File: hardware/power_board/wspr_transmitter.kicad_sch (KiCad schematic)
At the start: 3 parts, among them J6 Conn_Coaxial_Small, J7 Conn_Coaxial_Small, Y2 Si5351A-B-GT

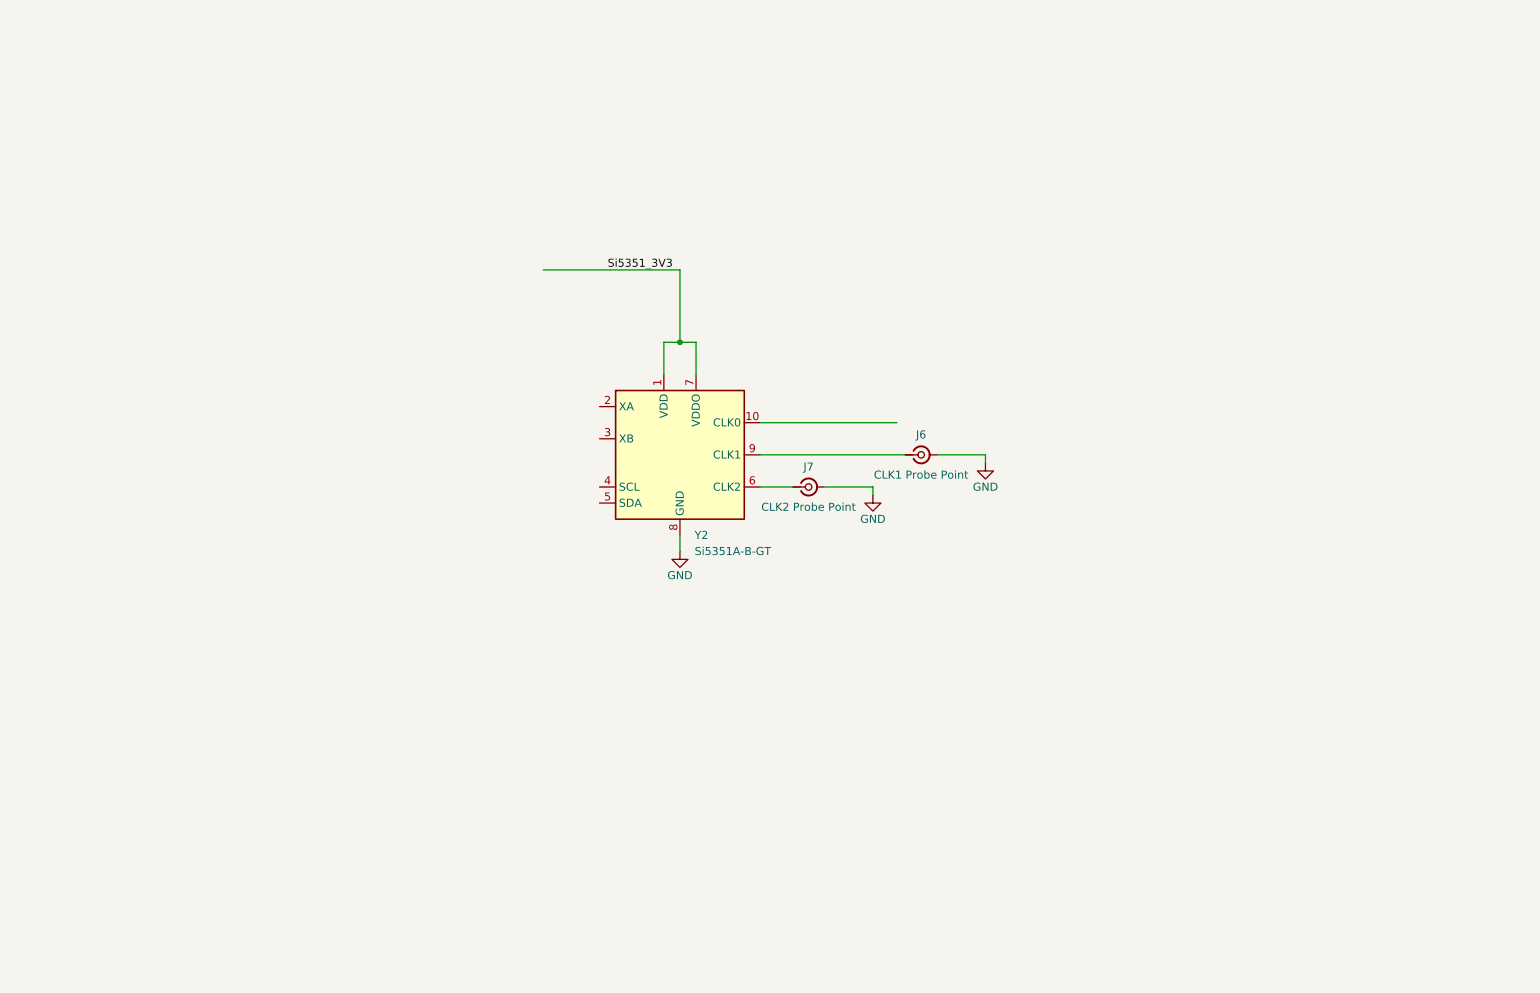
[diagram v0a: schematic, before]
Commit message: sync
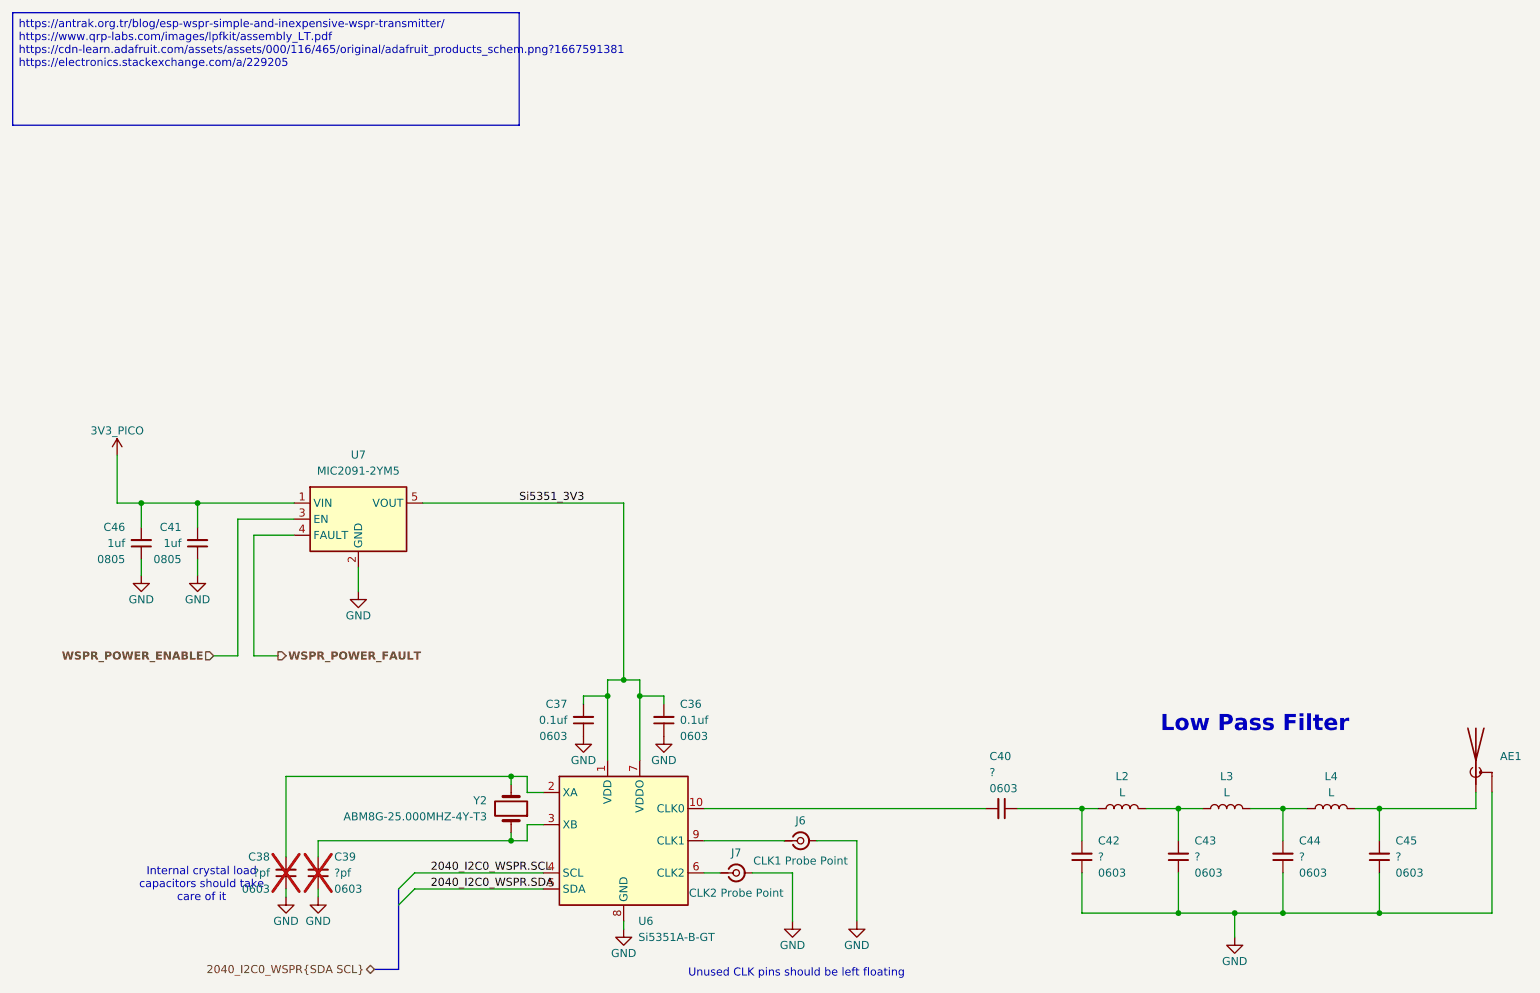
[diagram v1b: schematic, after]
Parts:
- added AE1: ~, giraffe_flight_computer_footprints:LINX_CONSMA001-G, symbol a_giraffe_symbols:Antenna_Shield
- added C36, C37: 0.1uf, Capacitor_SMD:C_0603_1608Metric_Pad1.08x0.95mm_HandSolder, symbol Device:C_Small
- added C38, C39: ?pf, Capacitor_SMD:C_0603_1608Metric_Pad1.08x0.95mm_HandSolder, symbol Device:C_Small
- added C40, C42, C43, C44, C45: ?, Capacitor_SMD:C_0603_1608Metric_Pad1.08x0.95mm_HandSolder, symbol Device:C_Small
- added C41, C46: 1uf, Capacitor_SMD:C_0603_1608Metric_Pad1.08x0.95mm_HandSolder, symbol Device:C_Small
- added L2, L3, L4: L, symbol Device:L
- added U7: MIC2091-2YM5, Package_TO_SOT_SMD:SOT-23-5, symbol Power_Management:MIC2091-2YM5
- added Y2: ABM8G-25.000MHZ-4Y-T3, symbol Device:Crystal
- renumbered Y2 to U6
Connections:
- net GND: now also AE1.2 (Shield), AE1.3 (Shield), AE1.4 (Shield), AE1.5 (Shield), C36.1, C37.1, C38.1, C39.1, C41.1, C42.1, C43.1, C44.1, C45.1, C46.1, U7.2 (GND)
- net Si5351_3V3: now also C36.2, C37.2, U7.5 (VOUT)
- net at U6.10 (CLK0): now also C40.2
- net at U6.2 (XA): now also C38.2, Y2.2
- net at U6.3 (XB): now also C39.2, Y2.1
- net 2040_I2C0_WSPR.SCL: now reaches U6.4 (SCL)
- net 2040_I2C0_WSPR.SDA: now reaches U6.5 (SDA)
- new net: AE1.1 (A), C45.2, L4.2
- new net: C43.2, L2.2, L3.1
- new net: C44.2, L3.2, L4.1
- new net: C40.1, C42.2, L2.1
- new net 3V3_PICO: C41.2, C46.2, U7.1 (VIN)
- new net WSPR_POWER_ENABLE: U7.3 (EN)
- new net WSPR_POWER_FAULT: U7.4 (FAULT)
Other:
- note added: "Internal crystal load capacitors should take care of it"
- note added: "Low Pass Filter"
- note added: "Unused CLK pins should be left floating"
- moved on the sheet: J6, J7, U6
